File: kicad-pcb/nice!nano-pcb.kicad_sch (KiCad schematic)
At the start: 14 parts, among them J1 Conn_Coaxial, SW1 SW_Push, SW2 SW_Push, SW3 SW_Nidec_CAS-120A1, U1 nice_nano, U2 LoRa-E220-900M22S

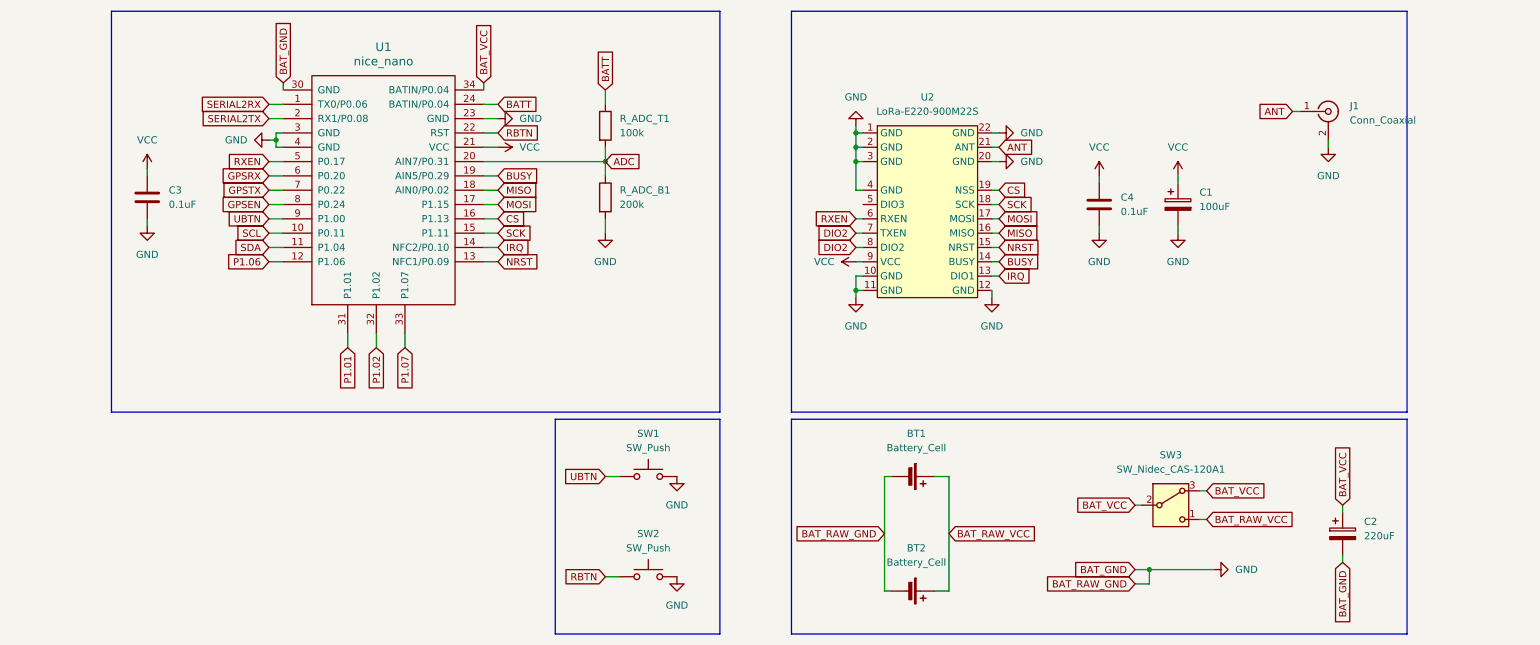
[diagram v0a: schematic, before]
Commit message: Final edits
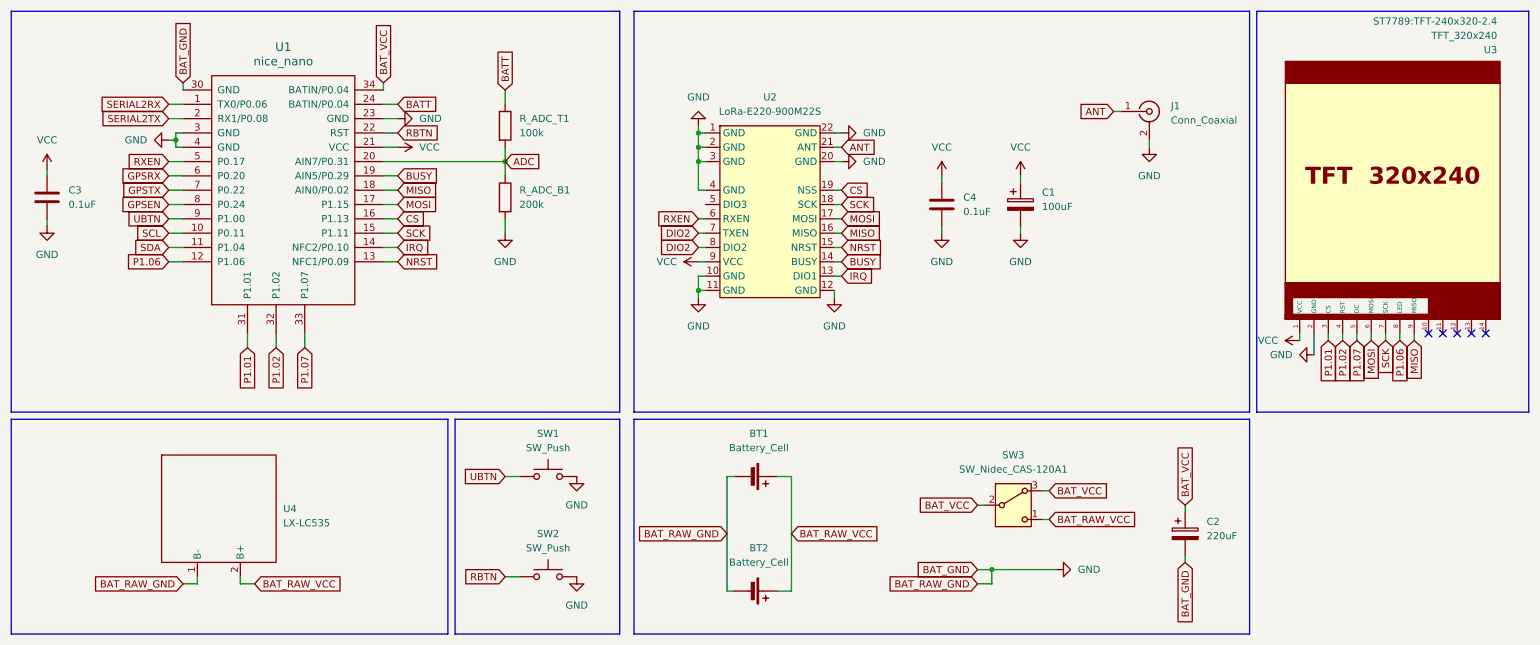
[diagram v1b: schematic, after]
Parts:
- added U3: TFT_320x240, ST7789:TFT-240x320-2.4, symbol ST7789:TFT_320x240
- added U4: LX-LC535, LX-LC535:LX-LC535, symbol LX-LC535:LX-LC535
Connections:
- net BAT_RAW_VCC: now also U4.2 (B+)
- net GND: now also U3.2 (GND), U4.1 (B-)
- net MISO: now also U3.9 (MISO)
- net MOSI: now also U3.6 (MOSI)
- net P1.01: now also U3.3 (CS)
- net P1.02: now also U3.4 (RST)
- net P1.06: now also U3.8 (LED)
- net P1.07: now also U3.5 (DC)
- net SCK: now also U3.7 (SCK)
- net VCC: now also U3.1 (VCC)
- no-connect marks 0 -> 5
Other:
- moved on the sheet: BT1, BT2, C1, C2, C3, C4, J1, R_ADC_B1, R_ADC_T1, SW1, SW2, SW3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
